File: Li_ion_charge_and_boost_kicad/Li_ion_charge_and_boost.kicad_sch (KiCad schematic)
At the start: 15 parts, among them U1 TP4056, U2 Type_C_6_pin, U3 DW01A

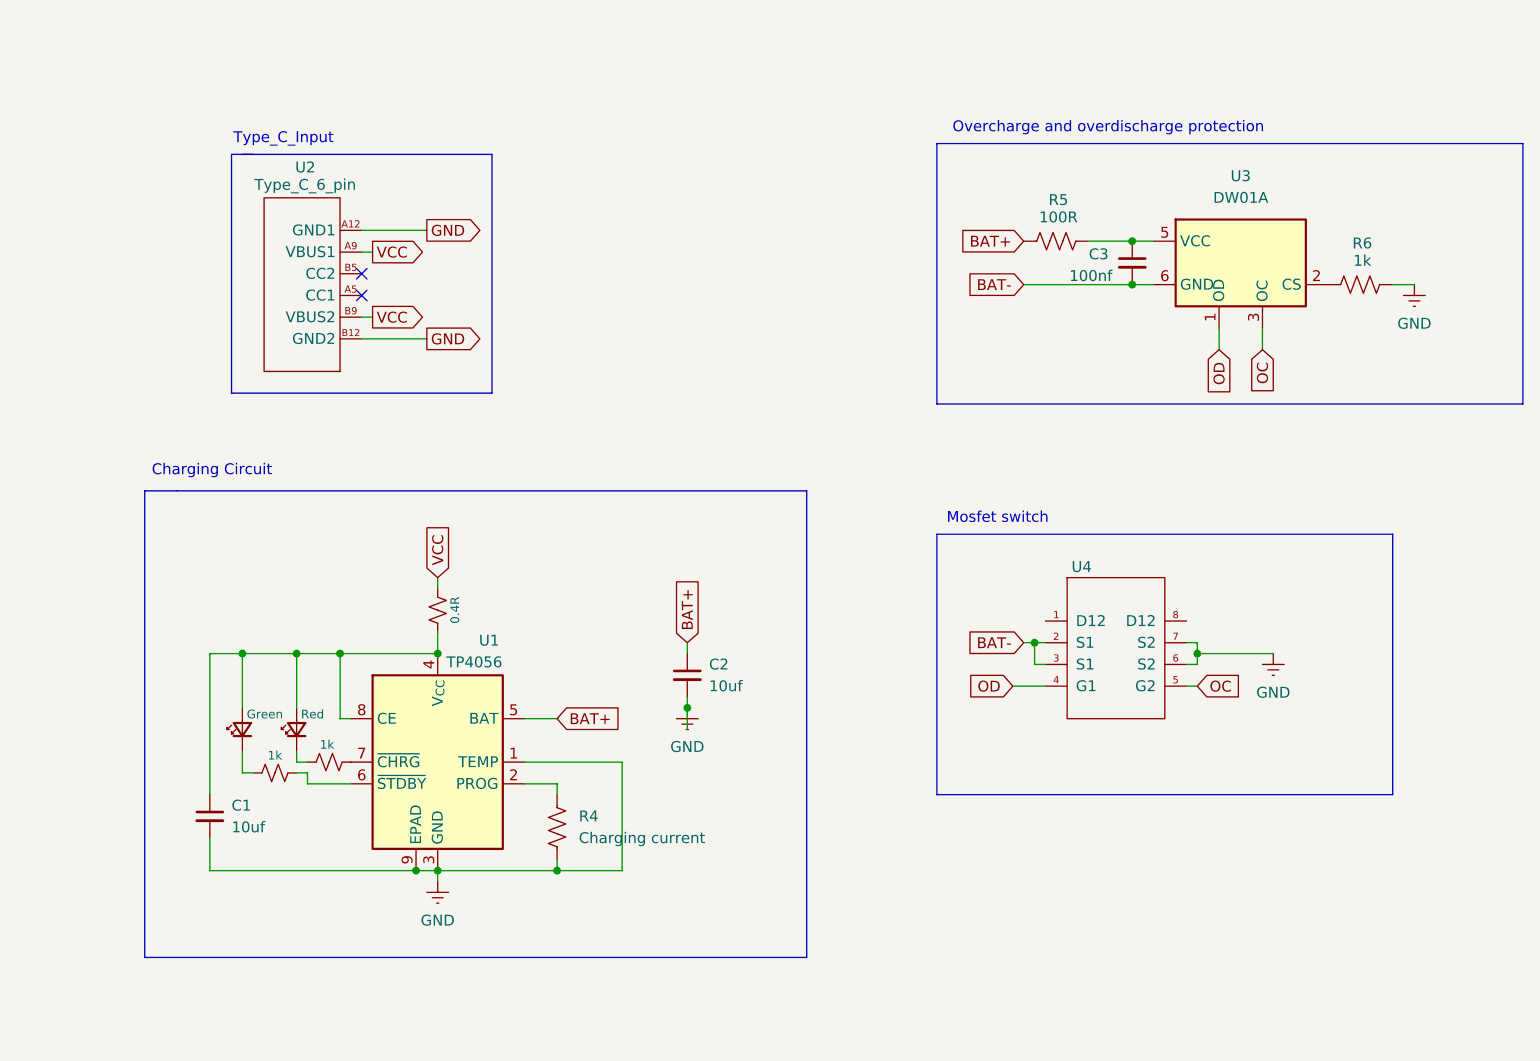
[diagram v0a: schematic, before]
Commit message: Li ion charger completed
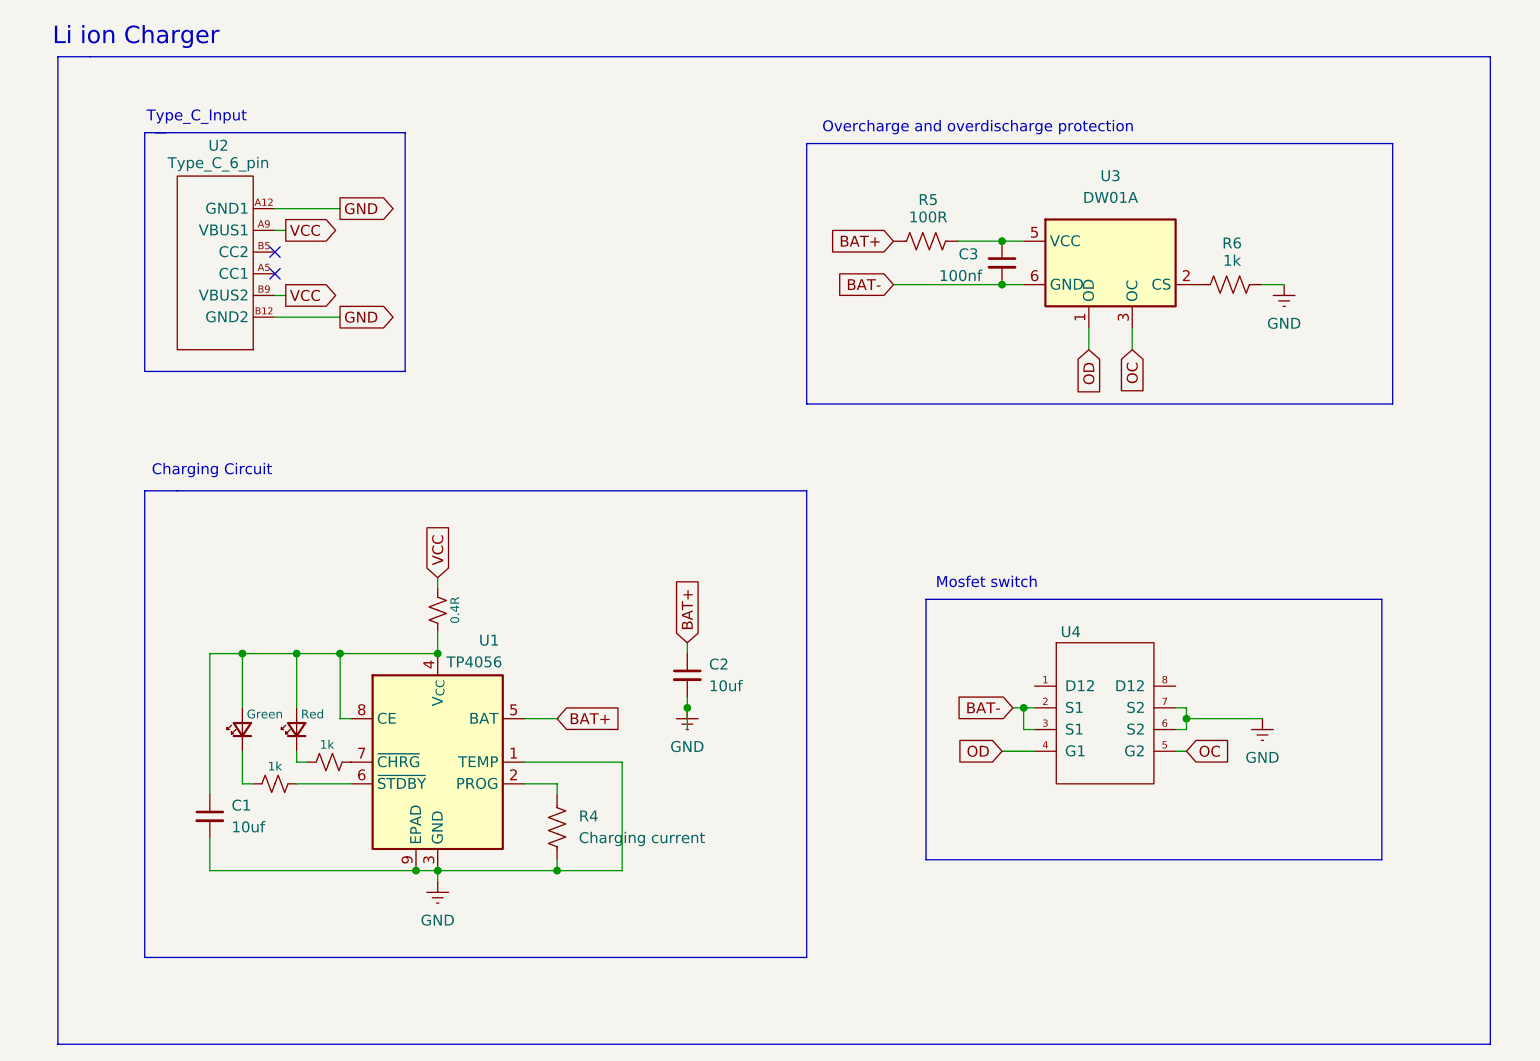
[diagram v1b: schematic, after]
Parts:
- U4: footprint (none) -> My Library:FS8205A
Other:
- note added: "Li ion Charger"
- moved on the sheet: C3, R5, R6, U2, U3, U4
